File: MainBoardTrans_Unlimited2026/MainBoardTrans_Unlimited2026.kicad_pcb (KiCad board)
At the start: 2 copper layers, 100 x 90 mm, 64 parts, among them J10 DSN-MINI-360, J11 pin_H, J12 RST, J13 I2C, J14 RJ45_Shielded, J15 Solenoid, J6 molex, J7 xt30, J8 Tblock, J9 ID-BAT, Q1 IRFZ44N, U1 TA6586, U10 TA6586, U2 TA6586, U3 TA6586, U4 TA6586, U5 TA6586, U6 ESP32-S3-DEVKITC-1, U7 ACS712xLCTR-05B, U8 BNO085, U9 AMS1117-3.3

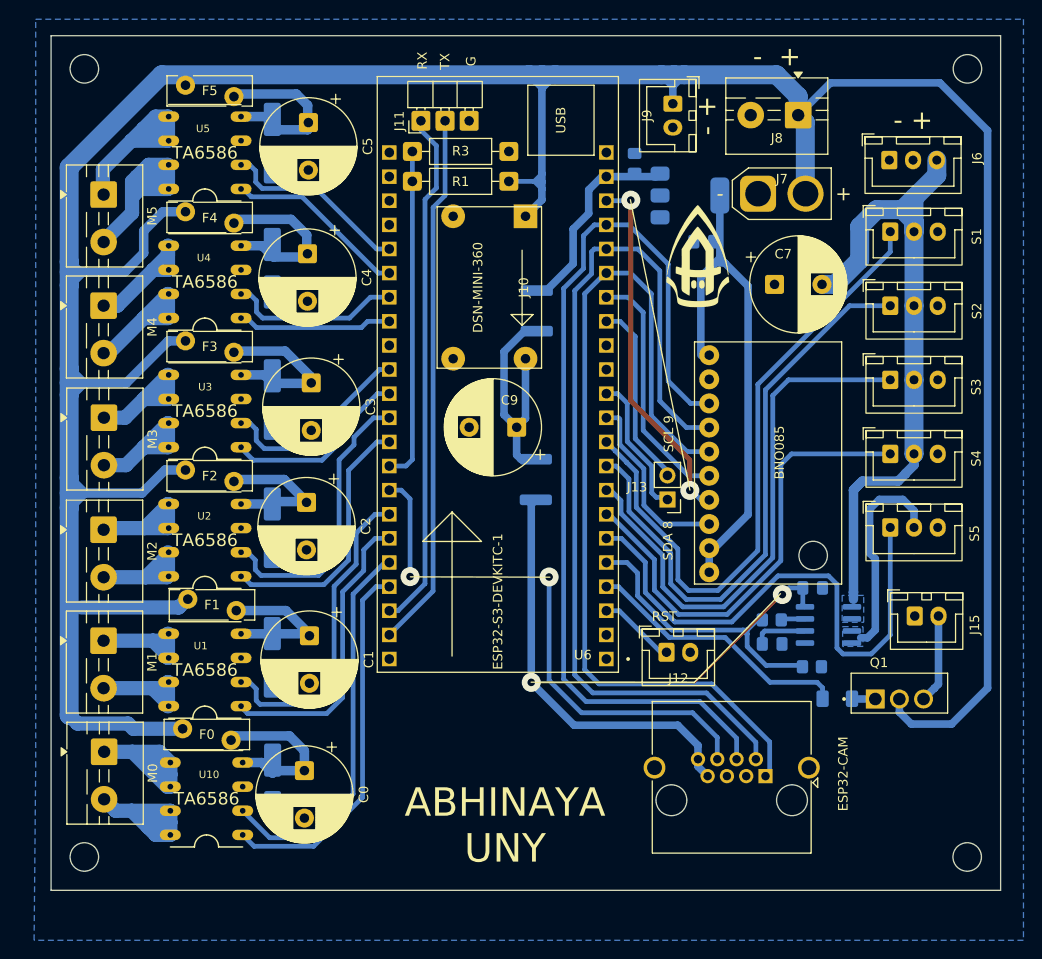
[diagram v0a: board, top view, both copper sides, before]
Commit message: Update PCB
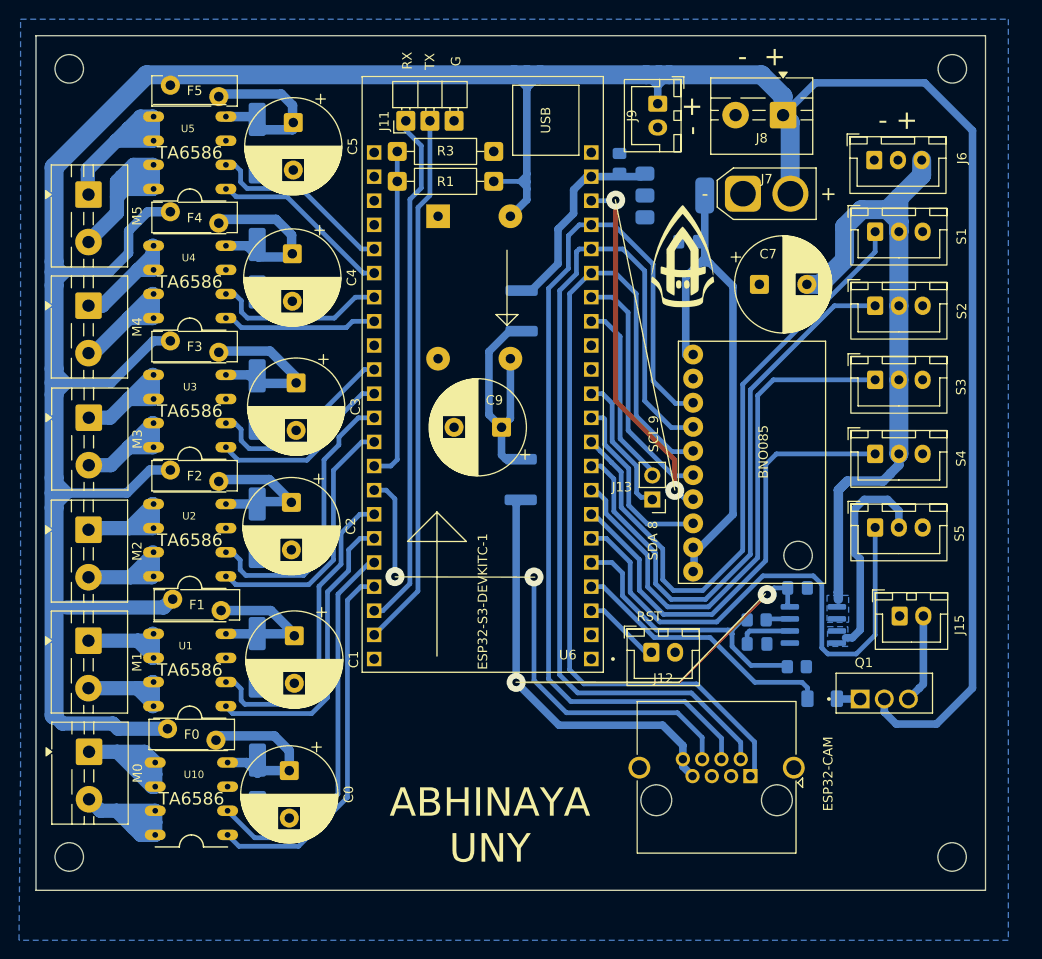
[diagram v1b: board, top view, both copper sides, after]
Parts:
- J10: moved to B.Cu
- moved U8 1.69 mm to (226.0, 60.5)
- moved C13 1.59 mm to (232.8, 91.0)
- moved C5 1.59 mm to (183.9, 36.1)
- moved J13 1.59 mm to (221.7, 75.8)
- moved M3 1.59 mm to (162.4, 67.2)
- moved R4 1.59 mm to (237.0, 93.4)
- moved S1 1.59 mm to (245.2, 47.6)
- moved S2 1.59 mm to (245.2, 55.4)
- moved C0 1.59 mm to (183.5, 104.3)
- moved C1 1.59 mm to (184.0, 90.1)
- moved C10 1.59 mm to (237.0, 85.1)
- moved C2 1.59 mm to (183.7, 76.1)
- moved C3 1.59 mm to (184.2, 63.5)
- moved C4 1.59 mm to (183.8, 49.9)
- moved C6 1.59 mm to (218.3, 40.4)
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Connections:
- C9 pad 1: Net-(J10-Pin_3) -> Net-(J10-Pin_4)
- F6 pad 1: Net-(J10-Pin_3) -> Net-(J10-Pin_4)
- F7 pad 1: Net-(J10-Pin_3) -> Net-(J10-Pin_4)
- J10 pad 1: +12V -> GND
- J10 pad 2: GND -> +12V
- J10 pad 3: Net-(J10-Pin_3) -> GND
- J10 pad 4: GND -> Net-(J10-Pin_4)
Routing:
- net Net-(J10-Pin_3): track 26.1 -> 0.00 mm
- net Net-(J10-Pin_4): track 0.00 -> 26.1 mm
